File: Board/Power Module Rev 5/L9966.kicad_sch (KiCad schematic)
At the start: 32 parts, among them U2 L9966CB-TR

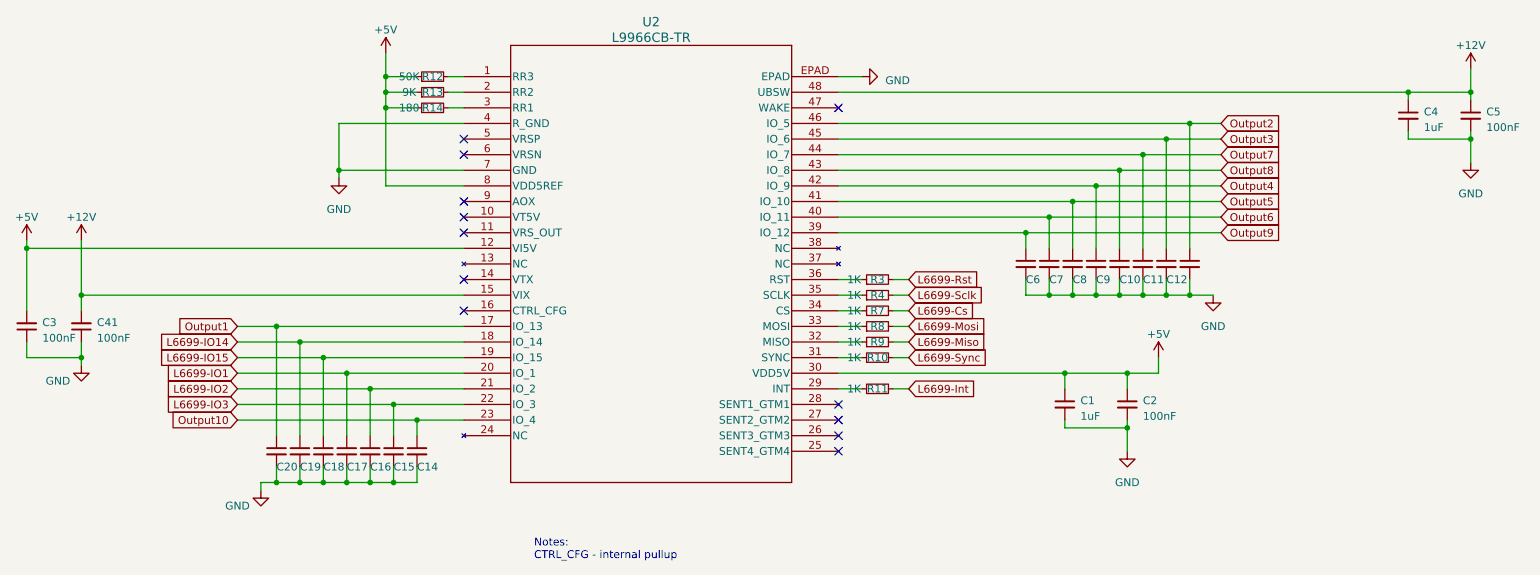
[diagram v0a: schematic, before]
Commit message: Update Board
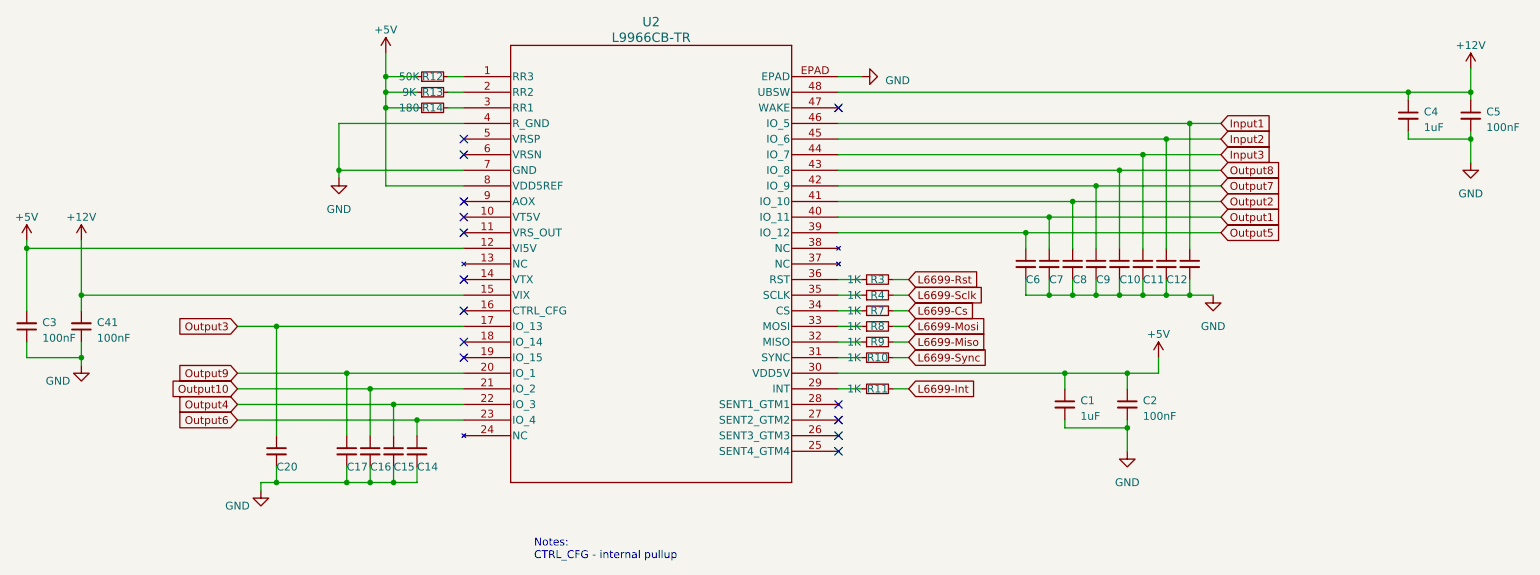
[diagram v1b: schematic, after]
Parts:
- removed C18, C19: 6.8nF, Capacitor_SMD:C_0603_1608Metric_Pad1.08x0.95mm_HandSolder, symbol Device:C_Small
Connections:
- net L6699-IO1 is gone; now on net Output9: C17.1, U2.20 (IO_1)
- net L6699-IO2 is gone; now on net Output10: C16.1, U2.21 (IO_2)
- net L6699-IO3 is gone; now on net Output4: C15.1, U2.22 (IO_3)
- net Output1: now also C7.1, U2.40 (IO_11); no longer C20.1, U2.17 (IO_13)
- net Output10: no longer C14.1, U2.23 (IO_4)
- net Output2: now also C8.1, U2.41 (IO_10); no longer C13.1, U2.46 (IO_5)
- net Output3: now also C20.1, U2.17 (IO_13); no longer C12.1, U2.45 (IO_6)
- net Output4: no longer C9.1, U2.42 (IO_9)
- net Output5: now also C6.1, U2.39 (IO_12); no longer C8.1, U2.41 (IO_10)
- net Output6: now also C14.1, U2.23 (IO_4); no longer C7.1, U2.40 (IO_11)
- net Output7: now also C9.1, U2.42 (IO_9); no longer C11.1, U2.44 (IO_7)
- net Output9: no longer C6.1, U2.39 (IO_12)
- net L6699-IO14: no longer names the net of U2.18 (IO_14)
- net L6699-IO15: no longer names the net of U2.19 (IO_15)
- new net Input1: C13.1, U2.46 (IO_5)
- new net Input2: C12.1, U2.45 (IO_6)
- new net Input3: C11.1, U2.44 (IO_7)
- no-connect marks 12 -> 14
